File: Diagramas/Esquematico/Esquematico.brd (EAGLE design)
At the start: 64 x 80 mm, 48 parts, among them IC3 DS3231N_DIP, IC4 3071_SMD, J1 Modulo Pir, J2 RASPBERRYPI-40-PIN-GPIO_SMT, K1 SRD-05VDC-SL-C, K2 SRD-05VDC-SL-C, K3 SRD-05VDC-SL-C, K4 SRD-05VDC-SL-C, U1 RFM69HW-868S2

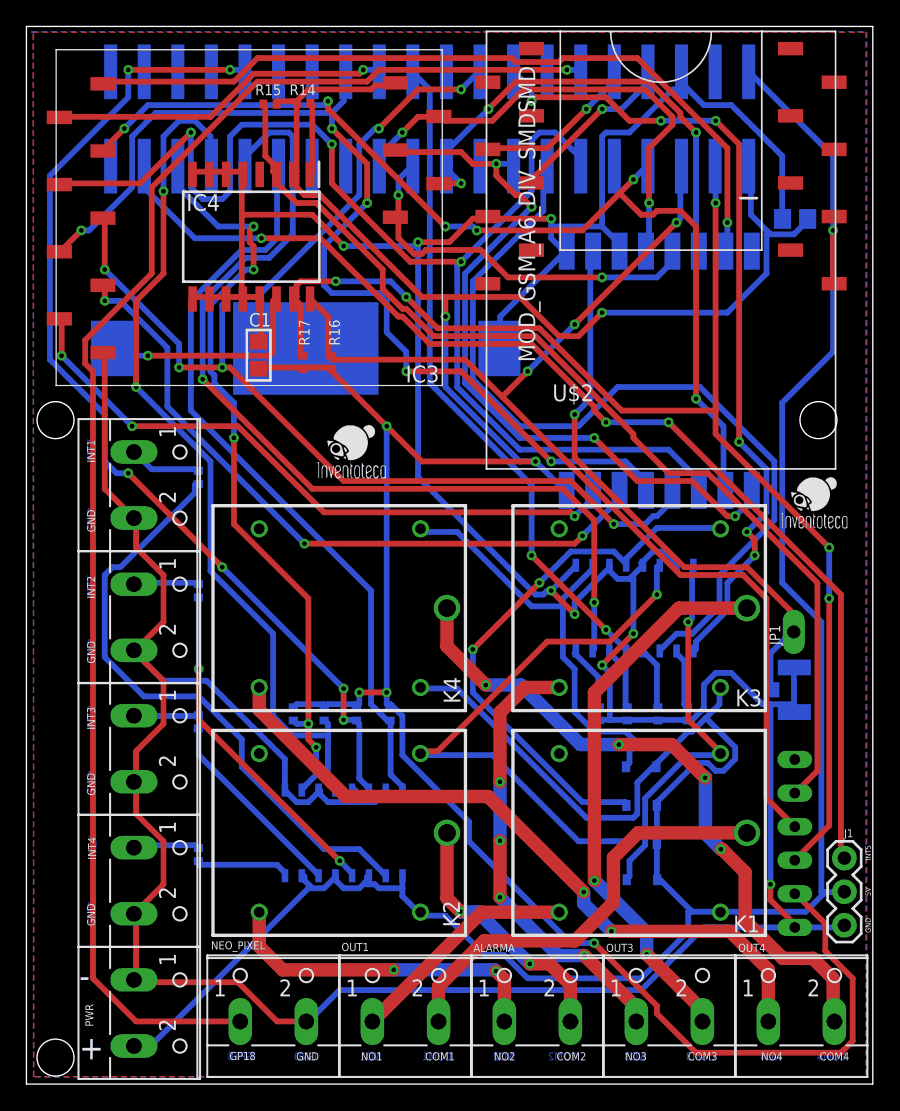
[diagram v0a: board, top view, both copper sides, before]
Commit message: Pcb "Terminado"
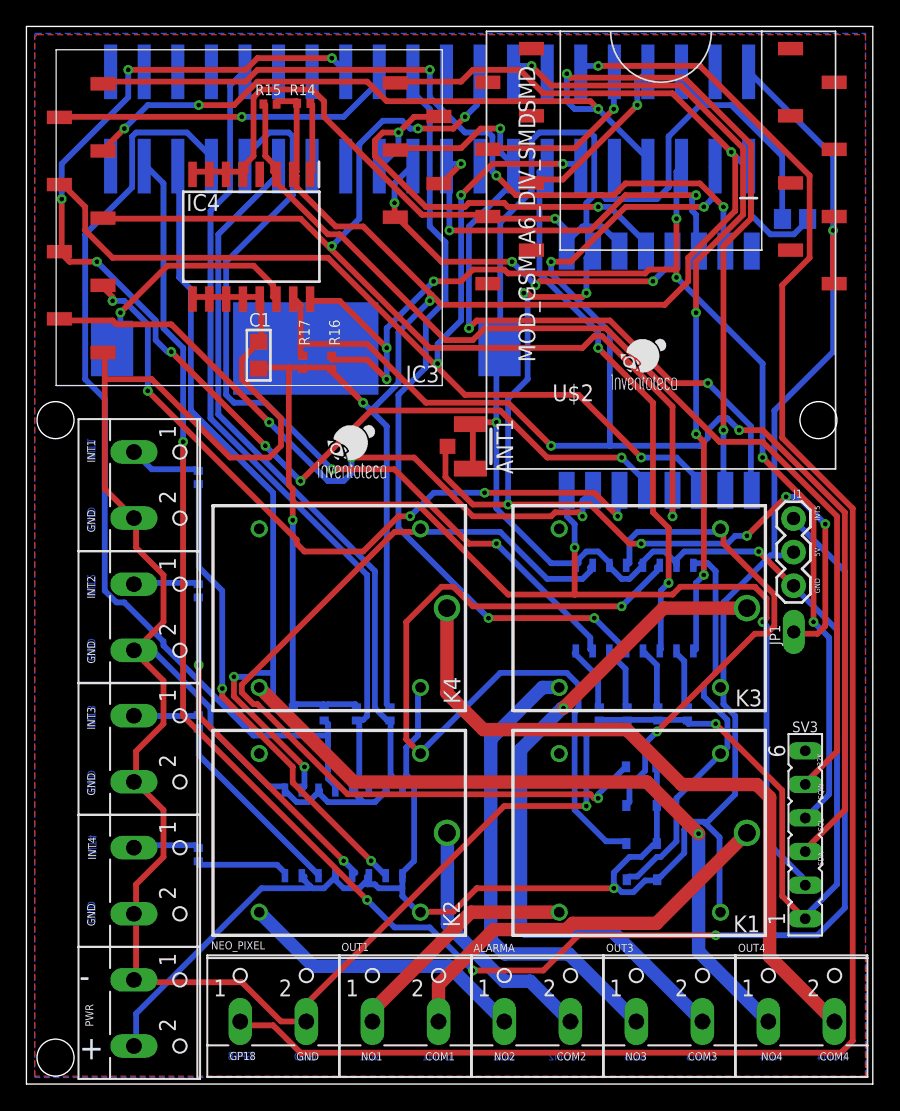
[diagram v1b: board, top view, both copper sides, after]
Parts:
- moved ANT1 30.6 mm to (33.6, 48.2), flipped to the top, turned to 270 degrees
- moved J1 26.0 mm to (58.0, 37.7)
- moved SV3 1.03 mm to (58.9, 18.9), flipped to the top
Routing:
- net INT5: track 87.4 -> 133.9 mm, vias 3 -> 4
- net N$32: track 33.3 -> 67.8 mm, vias 0 -> 1
- net GND: track 339.7 -> 373.7 mm, vias 8 -> 5
- net 5V: track 195.8 -> 163.1 mm, vias 1 -> 2
- net 3.3V: track 206.8 -> 238.9 mm, vias 7 -> 6
- net ANT_LORA: track 44.3 -> 71.1 mm, vias 1 -> 7
- net G18: track 110.8 -> 137.2 mm
- net OUT_ALARMA: track 65.0 -> 41.3 mm, vias 0 -> 2
- net N$34: track 43.7 -> 62.2 mm
- net G0: track 77.2 -> 94.3 mm, vias 6 -> 5
- net INT2: track 76.8 -> 61.3 mm, vias 6 -> 0
- net SDA: track 98.9 -> 112.7 mm, vias 5 -> 4
- net G1: track 95.7 -> 83.3 mm, vias 3 -> 4
- net G3: track 79.6 -> 90.7 mm, vias 5 -> 8
- net N$4: track 45.8 -> 35.5 mm, vias 0 -> 2
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
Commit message: Cambio de lugar
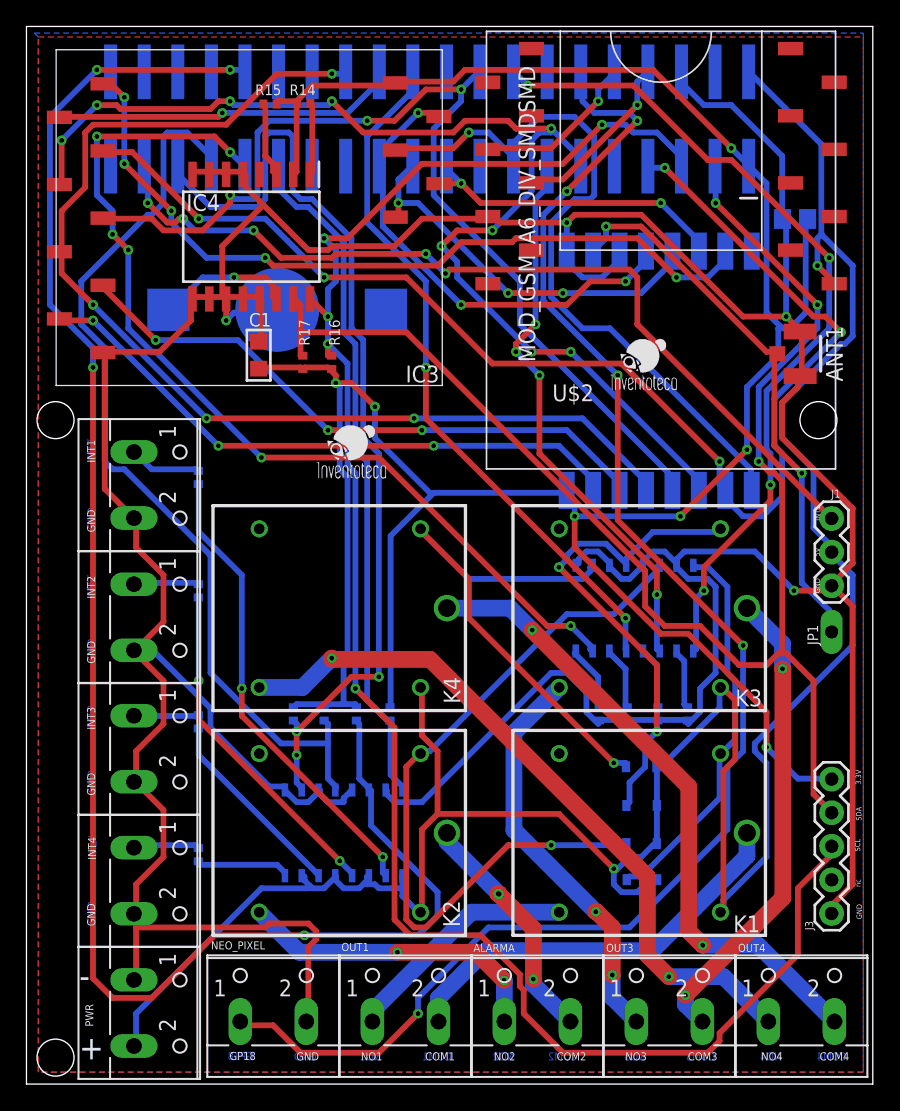
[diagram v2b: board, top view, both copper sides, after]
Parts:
- removed BT2: BU2032SM-BT-GTR, BU2032SM-BT-GTR:BAT_BU2032SM-BT-GTR
- removed SV3: (no value), con-lsta:FE06
- added B1: (no value), microbuilder:CR1220
- added J3: (no value), SparkFun-Connectors:1X05
- moved ANT1 25.9 mm to (58.5, 55.2)
- moved J1 2.88 mm to (60.9, 37.7)
- moved JP1 2.87 mm to (60.9, 34.2)
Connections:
- removed net 32K: SV3.6
- new net NC: J3.2
- net 3.3V: now also J3.5; no longer SV3.2
- net GND: now also B1.-, J3.1; no longer BT2.2, SV3.1
- net SCL: now also J3.3; no longer SV3.4
- net SDA: now also J3.4; no longer SV3.3
- net SQW: no longer SV3.5
- net VBAT: now also B1.+$1; no longer BT2.1
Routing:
- net SQW: track 81.3 -> 5.77 mm
- net INT2: track 61.3 -> 129.4 mm, vias 0 -> 4
- net INT5: track 133.9 -> 67.4 mm, vias 4 -> 5
- net SCL: track 95.2 -> 138.5 mm, vias 7 -> 5
- net GND: track 373.7 -> 337.6 mm, vias 5 -> 4
- net 3.3V: track 238.9 -> 203.4 mm, vias 6 -> 7
- net ANT_LORA: track 71.1 -> 42.2 mm, vias 7 -> 2
- net N$32: track 67.8 -> 40.2 mm
- net 5V: track 163.1 -> 188.8 mm
- net G18: track 137.2 -> 115.9 mm, vias 1 -> 5
- net COM3: track 51.7 -> 36.0 mm, vias 1 -> 2
- net INT4: track 59.6 -> 73.1 mm, vias 2 -> 3
- net OUT4: track 63.1 -> 73.0 mm, vias 2 -> 6
- net G4: track 55.2 -> 45.9 mm, vias 5 -> 3
- net MOSI: track 32.8 -> 24.1 mm, vias 3 -> 2
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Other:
- board text added: "nc"
- board text removed: "32K"
- board text removed: "SQW"
